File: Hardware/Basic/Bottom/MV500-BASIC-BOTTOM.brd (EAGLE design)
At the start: 33 x 33 mm, 32 parts, among them U1 AD5242-SO16

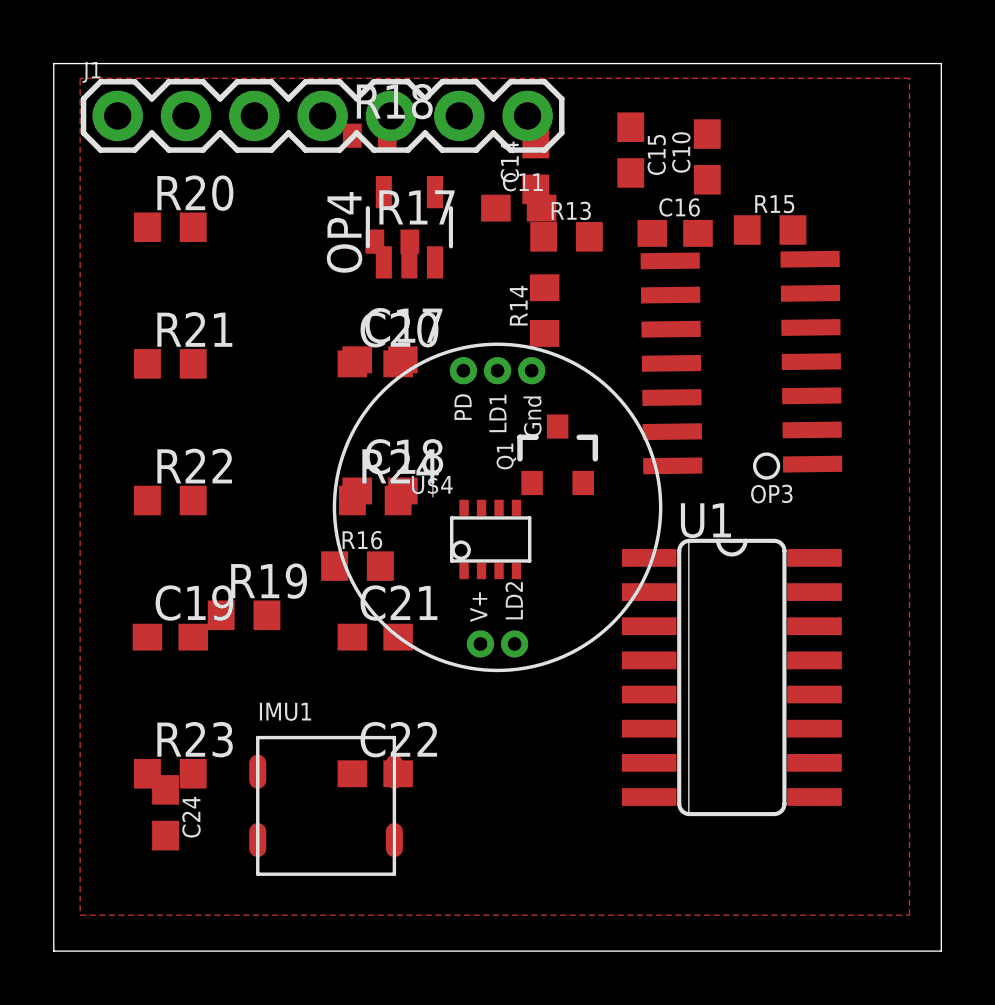
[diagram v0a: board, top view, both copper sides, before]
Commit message: Updated Bottom Board
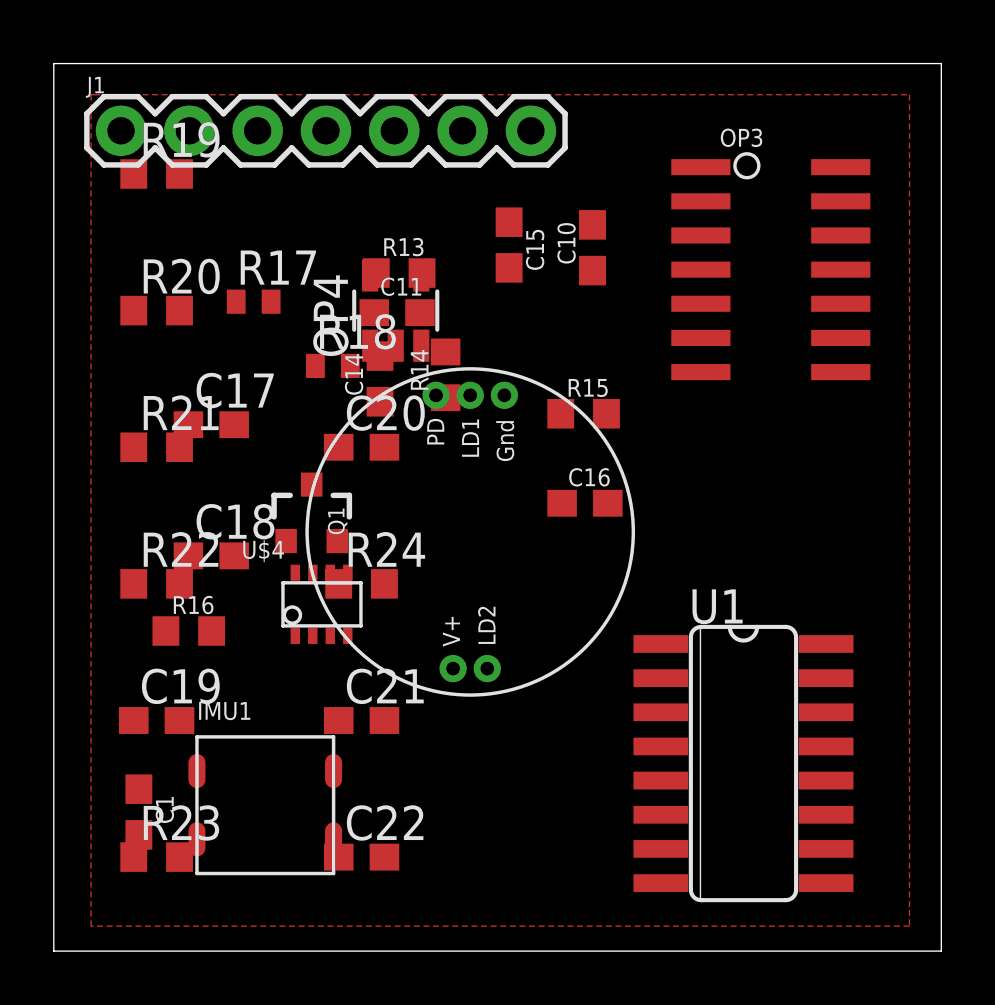
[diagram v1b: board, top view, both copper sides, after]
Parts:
- removed C24: 100n, LinnesLab-Passives:C0603
- added C1: 100n, LinnesLab-Passives:C0603
- moved R19 16.7 mm to (6.32, 31.4)
- moved C16 10.6 mm to (22.3, 19.2)
- moved C14 9.79 mm to (14.6, 23.8)
- moved R15 9.73 mm to (22.2, 22.5)
- moved Q1 9.40 mm to (12.1, 18.7)
- moved R18 8.67 mm to (12.9, 24.3)
- moved C17 6.72 mm to (8.36, 22.1)
- moved C18 6.72 mm to (8.36, 17.2)
- moved R16 6.72 mm to (7.52, 14.4)
- moved U$4 6.72 mm to (12.5, 15.4)
- moved R13 6.37 mm to (15.3, 27.7)
- moved C11 5.96 mm to (15.3, 26.2)
- moved C15 5.74 mm to (19.4, 28.8)
- moved R17 5.62 mm to (9.93, 26.6)
- moved C10 5.44 mm to (22.5, 28.7)
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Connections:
- net 3.3V: now also C1.2; no longer C24.2
- net GND: now also C1.1; no longer C24.1
